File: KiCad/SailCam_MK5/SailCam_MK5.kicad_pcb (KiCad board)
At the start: 4 copper layers, 65 x 65 mm, 70 parts, among them J1 B2B-PH-K-SLFSN, J2 B2B-PH-K-SLFSN, J3 B2B-PH-K-SLFSN, J4 B4B-PH-K-SLFSN, J5 SSW-108-02-G-S, J6 SSW-104-02-G-S, J7 USB_B, J8 DM3BT-DSF-PEJS, M1 2491, Q1 SS8050-G, Q2 SS8050-G, Q3 AOD1N60, U1 ADA4841-1YRZ-R7, U2 DS1672S-33+T&R, U3 NCV7805BD2TG, U4 LTC4054ES5-4.2#TRMPBF, U5 XC6220B331MR-G, U6 MAX485CSA+, U7 SM712.TCT, U8 CH340G, U9 MC74HC365ADG, Y1 ABS25-32.768KHZ-6-1-T, Y2 ECS-120-20-4X

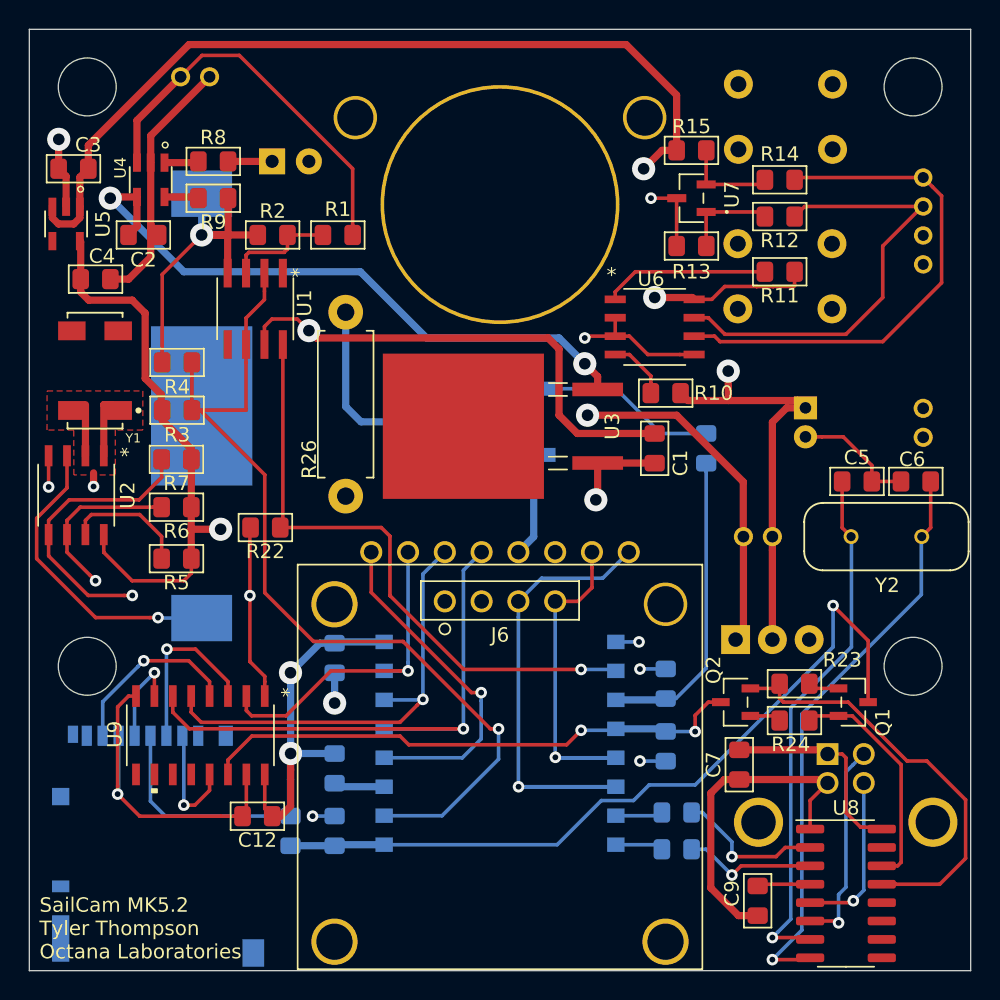
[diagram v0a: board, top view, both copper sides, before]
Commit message: mk5.2
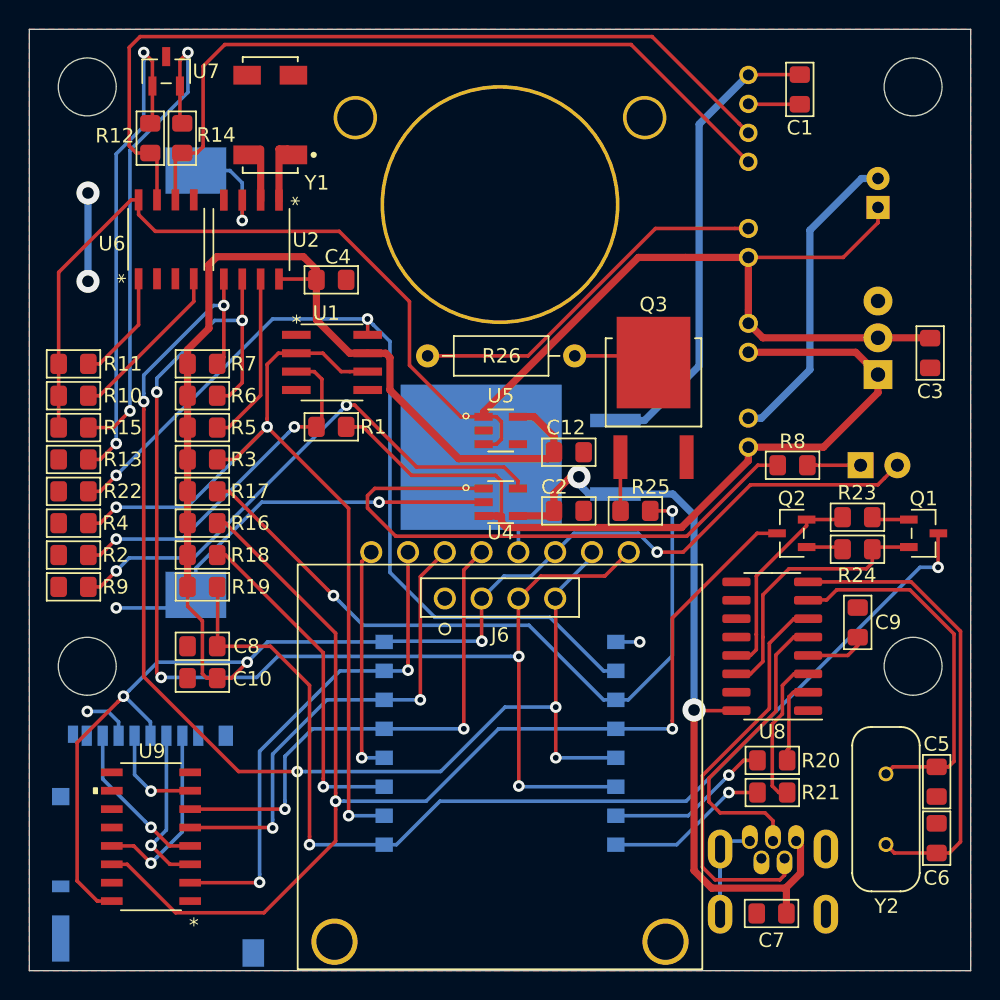
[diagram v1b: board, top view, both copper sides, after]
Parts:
- removed S2, S3: SW_Push, Button_Switch_THT:SW_PUSH_6mm
- added G***: LOGO, custom:octana_laboratories_logo, B.Cu at (147.6, 105.9)
- C10, C8, Q3, R16, R17, R18, R19, R20, R21, R25: moved to F.Cu
- J7: value USB_B -> USB_B_Mini; footprint footprints:AMPHENOL_61729-1011BLF -> digikey-footprints:USB_Mini_B_Female_548190519
- R26: footprint Resistor_THT:R_Axial_DIN0411_L9.9mm_D3.6mm_P12.70mm_Horizontal -> Resistor_THT:R_Axial_DIN0207_L6.3mm_D2.5mm_P10.16mm_Horizontal
- U3: moved to B.Cu
- moved C3 60.5 mm to (162.0, 85.8), turned to 90 degrees
- moved R11 49.2 mm to (102.9, 86.5), turned to 0 degrees
- moved R15 46.8 mm to (102.9, 90.9)
- moved D1 45.7 mm to (157.2, 93.5)
- moved R8 45.2 mm to (152.5, 93.5)
- moved R13 45.1 mm to (102.9, 93.1)
- moved J3 44.0 mm to (149.5, 90.3), turned to 90 degrees
- moved R12 43.8 mm to (108.2, 70.9), turned to 90 degrees
- moved R14 41.4 mm to (110.4, 70.9), turned to 90 degrees
- moved R10 40.9 mm to (102.9, 88.7), turned to 0 degrees
- moved U7 37.3 mm to (109.3, 66.3), turned to 0 degrees
- moved R16 35.5 mm to (111.8, 97.5), turned to 0 degrees
- moved C2 35.0 mm to (137.1, 96.7)
- moved R17 34.6 mm to (111.8, 95.3), turned to 0 degrees
- moved U6 34.3 mm to (109.3, 77.9), turned to 90 degrees
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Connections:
- C1 pad 1: VCC -> /CHG
- C1 pad 2: /CHG -> GND
- J7 pad 4: GND -> Net-(J7-Pad4)
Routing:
- net /Bat_Chg_Vcc: track 138.6 -> 55.3 mm
- net GND: track 144.6 -> 84.5 mm, vias 11 -> 6
- net VCC: track 205.3 -> 156.5 mm, vias 6 -> 4
- net Net-(R8-Pad1): track 2.38 -> 40.2 mm
- net /Vcc_5v_S: track 94.2 -> 57.7 mm, vias 1 -> 0
- net Net-(R9-Pad2): track 2.38 -> 37.5 mm, vias 0 -> 2
- net /Micro/RST: track 106.4 -> 76.3 mm, vias 1 -> 2
- net /Micro/GPIO2: track 21.3 -> 50.2 mm, vias 0 -> 2
- net Net-(R12-Pad2): track 6.80 -> 35.4 mm, vias 0 -> 2
- net Net-(R14-Pad2): track 6.80 -> 34.9 mm, vias 0 -> 2
- net /NEMA+: track 31.2 -> 57.7 mm
- net Net-(M1-Pad3): track 3.52 -> 23.6 mm, vias 0 -> 1
- net /OpAmpEN: track 42.4 -> 62.0 mm, vias 1 -> 2
- net /SD_CS: track 105.9 -> 87.2 mm
- net /Vcc_5v: track 124.6 -> 107.0 mm, vias 3 -> 0
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- removed copper zone on In1.Cu, net GND
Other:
- copper layers 4 -> 2
- board text added: "SailCam MK5.2 Tyler Thompson"
- board text removed: "SailCam MK5.2 Tyler Thompson Octana Laboratories"
